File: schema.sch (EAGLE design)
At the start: 22 parts, among them T1 2N2222, U1 ESP12E, X1 +5V

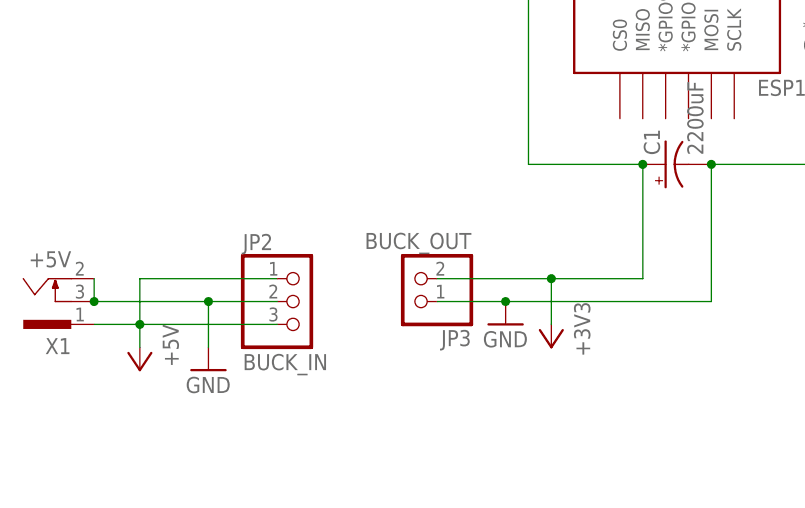
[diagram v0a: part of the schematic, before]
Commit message: Changed Buck
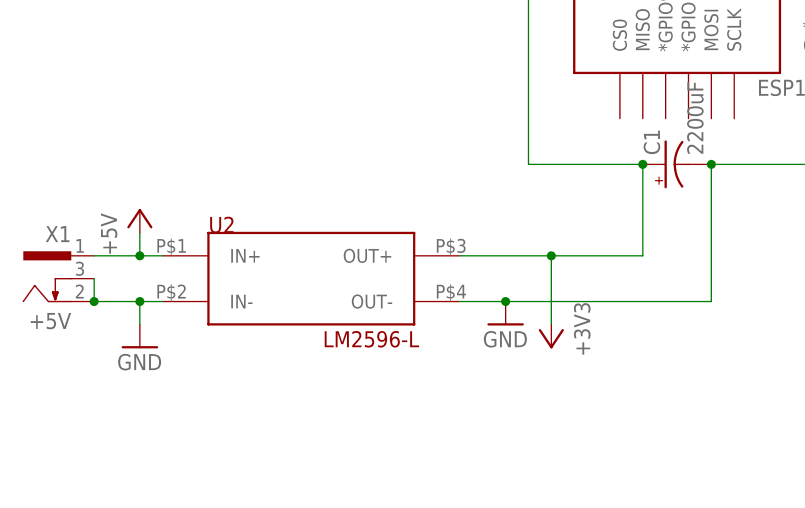
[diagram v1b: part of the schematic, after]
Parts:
- removed JP2: BUCK_IN, pinhead:PINHD-1X3
- removed JP3: BUCK_OUT, pinhead:PINHD-1X2
- added U2: LM2596-L, hi-link:LM2596-L
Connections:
- net +3V3: now also U2.OUT+; no longer JP3.2
- net +5V: now also U2.IN+; no longer JP2.1, JP2.3
- net GND: now also U2.IN-, U2.OUT-; no longer JP2.2, JP3.1
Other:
- moved on the sheet: X1
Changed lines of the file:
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@@
 <part name="GND7" library="supply1" deviceset="GND" device=""/>
 <part name="X1" library="con-conrad" deviceset="73398?" device="9-5" value="+5V"/>
-<part name="JP2" library="pinhead" deviceset="PINHD-1X3" device="" value="BUCK_IN"/>
 <part name="P+1" library="supply1" deviceset="+5V" device=""/>
 <part name="GND1" library="supply1" deviceset="GND" device=""/>
-<part name="JP3" library="pinhead" deviceset="PINHD-1X2" device="" value="BUCK_OUT"/>
 <part name="GND5" library="supply1" deviceset="GND" device=""/>
 <part name="C1" library="SparkFun-Capacitors" deviceset="100UF-25V-20%(PTH)" device="" value="2200uF"/>
@@
 <part name="GND4" library="supply1" deviceset="GND" device=""/>
 <part name="R1" library="pot" deviceset="TRIM_EU-" device="CA6V" value="14k"/>
+<part name="U2" library="hi-link" deviceset="LM2596-L" device=""/>
 </parts>
 <sheets>
@@
 <instance part="+3V35" gate="G$1" x="-58.42" y="261.62" rot="R180"/>
 <instance part="GND7" gate="1" x="-55.88" y="259.08"/>
-<instance part="X1" gate="G$1" x="-154.94" y="203.2" rot="R180"/>
-<instance part="JP2" gate="A" x="-127" y="203.2"/>
-<instance part="P+1" gate="1" x="-144.78" y="195.58" rot="R180"/>
-<instance part="GND1" gate="1" x="-137.16" y="195.58"/>
-<instance part="JP3" gate="G$1" x="-114.3" y="205.74" rot="R180"/>
+<instance part="X1" gate="G$1" x="-154.94" y="205.74" rot="MR0"/>
+<instance part="P+1" gate="1" x="-144.78" y="213.36"/>
+<instance part="GND1" gate="1" x="-144.78" y="198.12"/>
 <instance part="GND5" gate="1" x="-104.14" y="200.66"/>
 <instance part="C1" gate="G$1" x="-86.36" y="218.44" rot="R90"/>
@@
 <instance part="GND4" gate="1" x="-114.3" y="274.32"/>
 <instance part="R1" gate="1" x="-119.38" y="279.4" rot="MR180"/>
+<instance part="U2" gate="G$1" x="-127" y="205.74"/>
 </instances>
 <busses>
@@
 </segment>
 <segment>
-<pinref part="X1" gate="G$1" pin="3"/>
-<pinref part="X1" gate="G$1" pin="2"/>
-<wire x1="-149.86" y1="203.2" x2="-149.86" y2="205.74" width="0.1524" layer="91"/>
-<pinref part="JP2" gate="A" pin="2"/>
-<wire x1="-149.86" y1="203.2" x2="-137.16" y2="203.2" width="0.1524" layer="91"/>
-<pinref part="GND1" gate="1" pin="GND"/>
-<wire x1="-137.16" y1="203.2" x2="-129.54" y2="203.2" width="0.1524" layer="91"/>
-<wire x1="-137.16" y1="198.12" x2="-137.16" y2="203.2" width="0.1524" layer="91"/>
-<junction x="-137.16" y="203.2"/>
-<junction x="-149.86" y="203.2"/>
-</segment>
-<segment>
-<pinref part="JP3" gate="G$1" pin="1"/>
 <pinref part="GND5" gate="1" pin="GND"/>
-<wire x1="-111.76" y1="203.2" x2="-104.14" y2="203.2" width="0.1524" layer="91"/>
 <pinref part="U1" gate="G$1" pin="GND"/>
 <pinref part="C1" gate="G$1" pin="-"/>
+<wire x1="-109.22" y1="203.2" x2="-104.14" y2="203.2" width="0.1524" layer="91"/>
 <wire x1="-68.58" y1="241.3" x2="-68.58" y2="218.44" width="0.1524" layer="91"/>
 <wire x1="-68.58" y1="218.44" x2="-81.28" y2="218.44" width="0.1524" layer="91"/>
@@
 <junction x="-81.28" y="218.44"/>
 <junction x="-104.14" y="203.2"/>
+<pinref part="U2" gate="G$1" pin="OUT-"/>
 </segment>
 <segment>
@@
 <wire x1="-114.3" y1="276.86" x2="-114.3" y2="279.4" width="0.1524" layer="91"/>
 </segment>
+<segment>
+<pinref part="X1" gate="G$1" pin="3"/>
+<pinref part="X1" gate="G$1" pin="2"/>
+<wire x1="-149.86" y1="205.74" x2="-149.86" y2="203.2" width="0.1524" layer="91"/>
+<pinref part="U2" gate="G$1" pin="IN-"/>
+<wire x1="-149.86" y1="203.2" x2="-144.78" y2="203.2" width="0.1524" layer="91"/>
+<junction x="-149.86" y="203.2"/>
+<pinref part="GND1" gate="1" pin="GND"/>
+<wire x1="-144.78" y1="203.2" x2="-142.24" y2="203.2" width="0.1524" layer="91"/>
+<wire x1="-144.78" y1="200.66" x2="-144.78" y2="203.2" width="0.1524" layer="91"/>
+<junction x="-144.78" y="203.2"/>
+</segment>
 </net>
 <net name="+3V3" class="0">
@@
 </segment>
 <segment>
-<pinref part="JP3" gate="G$1" pin="2"/>
-<wire x1="-111.76" y1="205.74" x2="-99.06" y2="205.74" width="0.1524" layer="91"/>
 <pinref part="U1" gate="G$1" pin="VCC"/>
 <pinref part="C1" gate="G$1" pin="+"/>
-<wire x1="-99.06" y1="205.74" x2="-88.9" y2="205.74" width="0.1524" layer="91"/>
+<wire x1="-99.06" y1="208.28" x2="-88.9" y2="208.28" width="0.1524" layer="91"/>
 <wire x1="-101.6" y1="241.3" x2="-101.6" y2="218.44" width="0.1524" layer="91"/>
 <wire x1="-101.6" y1="218.44" x2="-88.9" y2="218.44" width="0.1524" layer="91"/>
-<wire x1="-88.9" y1="218.44" x2="-88.9" y2="205.74" width="0.1524" layer="91"/>
+<wire x1="-88.9" y1="218.44" x2="-88.9" y2="208.28" width="0.1524" layer="91"/>
 <junction x="-88.9" y="218.44"/>
 <pinref part="+3V34" gate="G$1" pin="+3V3"/>
-<wire x1="-99.06" y1="200.66" x2="-99.06" y2="205.74" width="0.1524" layer="91"/>
-<junction x="-99.06" y="205.74"/>
+<wire x1="-99.06" y1="200.66" x2="-99.06" y2="208.28" width="0.1524" layer="91"/>
+<pinref part="U2" gate="G$1" pin="OUT+"/>
+<wire x1="-99.06" y1="208.28" x2="-109.22" y2="208.28" width="0.1524" layer="91"/>
+<junction x="-99.06" y="208.28"/>
 </segment>
 </net>
@@
 </net>
 <net name="+5V" class="0">
-<segment>
-<pinref part="X1" gate="G$1" pin="1"/>
-<wire x1="-149.86" y1="200.66" x2="-144.78" y2="200.66" width="0.1524" layer="91"/>
-<wire x1="-144.78" y1="200.66" x2="-144.78" y2="205.74" width="0.1524" layer="91"/>
-<pinref part="JP2" gate="A" pin="1"/>
-<wire x1="-129.54" y1="205.74" x2="-144.78" y2="205.74" width="0.1524" layer="91"/>
-<pinref part="JP2" gate="A" pin="3"/>
-<wire x1="-144.78" y1="200.66" x2="-129.54" y2="200.66" width="0.1524" layer="91"/>
-<pinref part="P+1" gate="1" pin="+5V"/>
-<wire x1="-144.78" y1="198.12" x2="-144.78" y2="200.66" width="0.1524" layer="91"/>
-<junction x="-144.78" y="200.66"/>
-</segment>
 <segment>
 <pinref part="D1" gate="G$1" pin="C"/>
@@
 <junction x="-35.56" y="203.2"/>
 </segment>
-</net>
+<segment>
+<pinref part="X1" gate="G$1" pin="1"/>
+<pinref part="U2" gate="G$1" pin="IN+"/>
+<wire x1="-149.86" y1="208.28" x2="-144.78" y2="208.28" width="0.1524" layer="91"/>
+<pinref part="P+1" gate="1" pin="+5V"/>
+<wire x1="-144.78" y1="208.28" x2="-142.24" y2="208.28" width="0.1524" layer="91"/>
+<wire x1="-144.78" y1="210.82" x2="-144.78" y2="208.28" width="0.1524" layer="91"/>
+<junction x="-144.78" y="208.28"/>
+</segment>
+</net>
